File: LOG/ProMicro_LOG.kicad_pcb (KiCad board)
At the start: 2 copper layers, 17.8 x 30.5 mm, 16 parts, among them J1 Micro_SD_Card_Det, U1 DS3231MZ

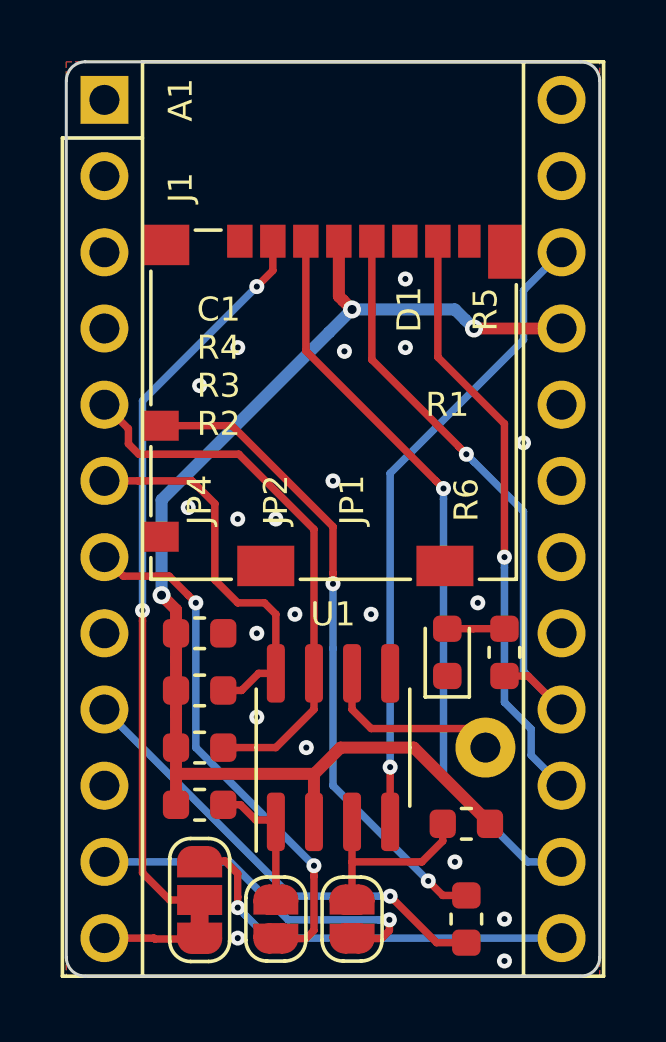
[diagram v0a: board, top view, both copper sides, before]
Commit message: dump
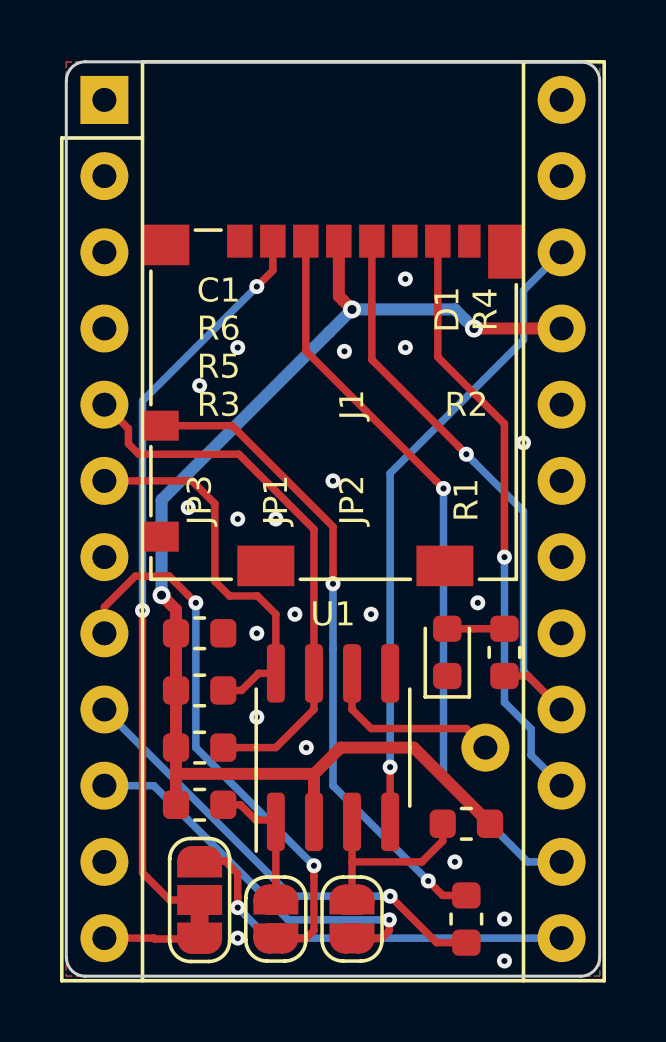
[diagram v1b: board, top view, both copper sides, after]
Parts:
- A1: value Sparkfun_Pro_Micro_3V3 -> Sparkfun_Pro_Micro
- moved LOGO1 10.2 mm to (144.8, 80.0)
- renumbered JP2 to JP1, JP1 to JP2, JP4 to JP3, R6 to R1, R1 to R2, R2 to R3, R5 to R4, R3 to R5, R4 to R6
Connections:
- net Reset renamed ~RST
- A1 pad 10: (no net) -> INT
- A1 pad 11: INT -> (no net)
- A1 pad 3: (no net) -> GND
- A1 pad 7: TRG -> (no net)
- A1 pad 8: (no net) -> PWM
- JP1 pad 2: TRG -> PWM
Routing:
- net PWM: track 0.00 -> 18.7 mm, vias 0 -> 2
- net TRG: track 17.6 -> 0.00 mm, vias 2 -> 0
- net INT: track 12.0 -> 13.1 mm
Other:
- board text added: "3V3"
- board text added: "BTN"
- board text added: "CIPO"
- board text added: "COPI"
- board text added: "CS0"
- board text added: "CS1"
- board text added: "GND"
- board text added: "INT"
- board text added: "PWM"
- board text added: "RST"
- board text added: "SCK"
- board text added: "SCL"
- board text added: "SDA"
- board text added: "VBAT"
- board text added: "nerdyscout.github.io/ ProMicro/LOG v1.2"
- board text removed: "nerdyscout.github.io/ProMicro/LOG"
- board text removed: "v1.1"

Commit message: clean
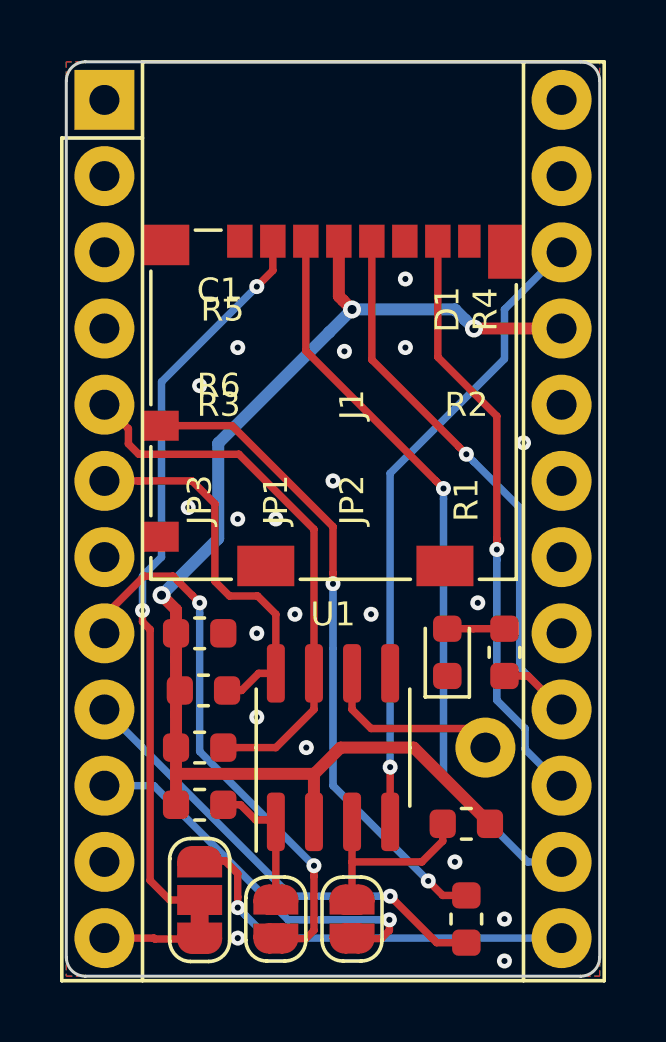
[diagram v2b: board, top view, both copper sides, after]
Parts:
- moved R5 1.91 mm to (140.5, 95.9)
- moved R6 1.91 mm to (140.3, 97.8)
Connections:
- R5 pad 2: SDA -> SCL
- R6 pad 2: SCL -> SDA
